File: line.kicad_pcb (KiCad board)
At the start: 2 copper layers, 68 parts, among them P1 CONN_01X08, P2 CONN_01X08, P3 CONN_01X03, P4 CONN_01X03, U1 TL072, U2 LM7805CT, U3 LM7905CT, U4 TL072

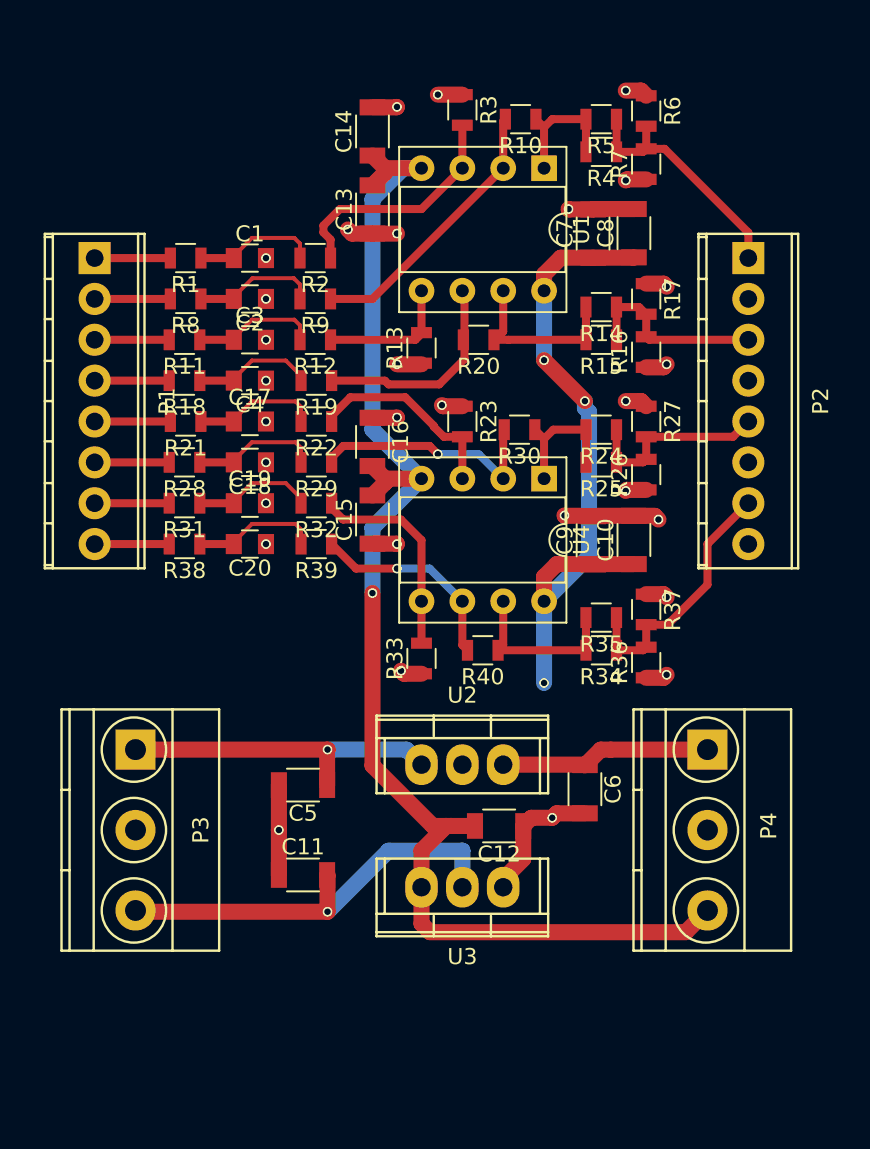
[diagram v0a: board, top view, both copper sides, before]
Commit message: line receiver PCB looks complete
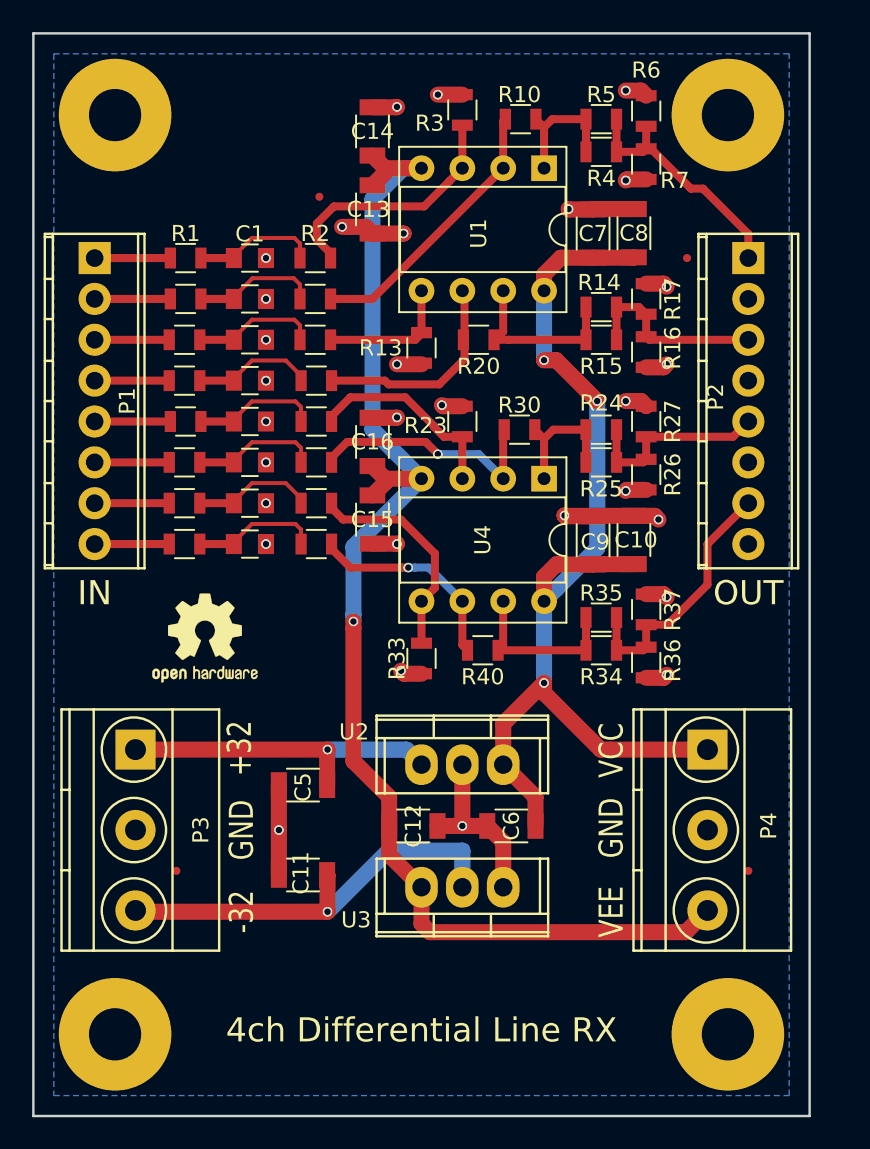
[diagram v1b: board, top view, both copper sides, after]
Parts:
- added FID1: FIDUCIAL, smd:FID0.5, F.Cu at (74.9, 36.8)
- added FID2: FIDUCIAL, smd:FID0.5, F.Cu at (97.8, 40.6)
- added FID3: FIDUCIAL, smd:FID0.5, F.Cu at (66.0, 78.7)
- added FID4: FIDUCIAL, smd:FID0.5, F.Cu at (101.6, 78.7)
- added REF**: hole3mm, pcb:hole3mm, F.Cu at (100.3, 88.9)
- added REF**: hole3mm, pcb:hole3mm, F.Cu at (62.2, 88.9)
- added REF**: hole3mm, pcb:hole3mm, F.Cu at (62.2, 31.8)
- added REF**: hole3mm, pcb:hole3mm, F.Cu at (100.3, 31.8)
- added REF***: OSHW-Logo2_7.3x6mm_Copper, Symbols:OSHW-Logo2_7.3x6mm_Copper, F.Cu at (67.8, 64.3)
- added REF***: OSHW-Logo2_7.3x6mm_SilkScreen, Symbols:OSHW-Logo2_7.3x6mm_SilkScreen, F.Cu at (67.8, 64.3)
- moved C12 5.33 mm to (80.8, 75.9)
- moved C6 5.11 mm to (86.9, 75.9), turned to 180 degrees
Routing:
- net /VCC: track 54.3 -> 65.1 mm
- net GND: track 48.3 -> 54.1 mm
- net /VEE: track 85.1 -> 82.5 mm
- net Net-(R32-Pad1): track 13.1 -> 13.8 mm
- added copper zone on B.Cu, net GND
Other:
- board outline added: 48.3 x 67.3 mm
- board text added: "+32"
- board text added: "-32"
- board text added: "4ch Differential Line RX"
- board text added: "A"
- board text added: "A+"
- board text added: "A-"
- board text added: "B"
- board text added: "B+"
- board text added: "B-"
- board text added: "C"
- board text added: "C+"
- board text added: "C-"
- board text added: "D"
- board text added: "D+"
- board text added: "D-"
- board text added: "GND"
- board text added: "IN"
- board text added: "Inputs"
- board text added: "OUT"
- board text added: "Outputs"
- board text added: "Rev.A 201710"
- board text added: "VCC"
- board text added: "VEE"
- board text added: "github.com/phenidone"
- board text added: "william@brodie-tyrrell.org"
